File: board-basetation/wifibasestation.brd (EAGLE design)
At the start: 50 x 22 mm, 33 parts, among them IC1 1117EMP, IC2 HTU21D, J1 SWD_SHROUD_SMD, X1 ESP-03, X2 SMA-142-0711-821/826

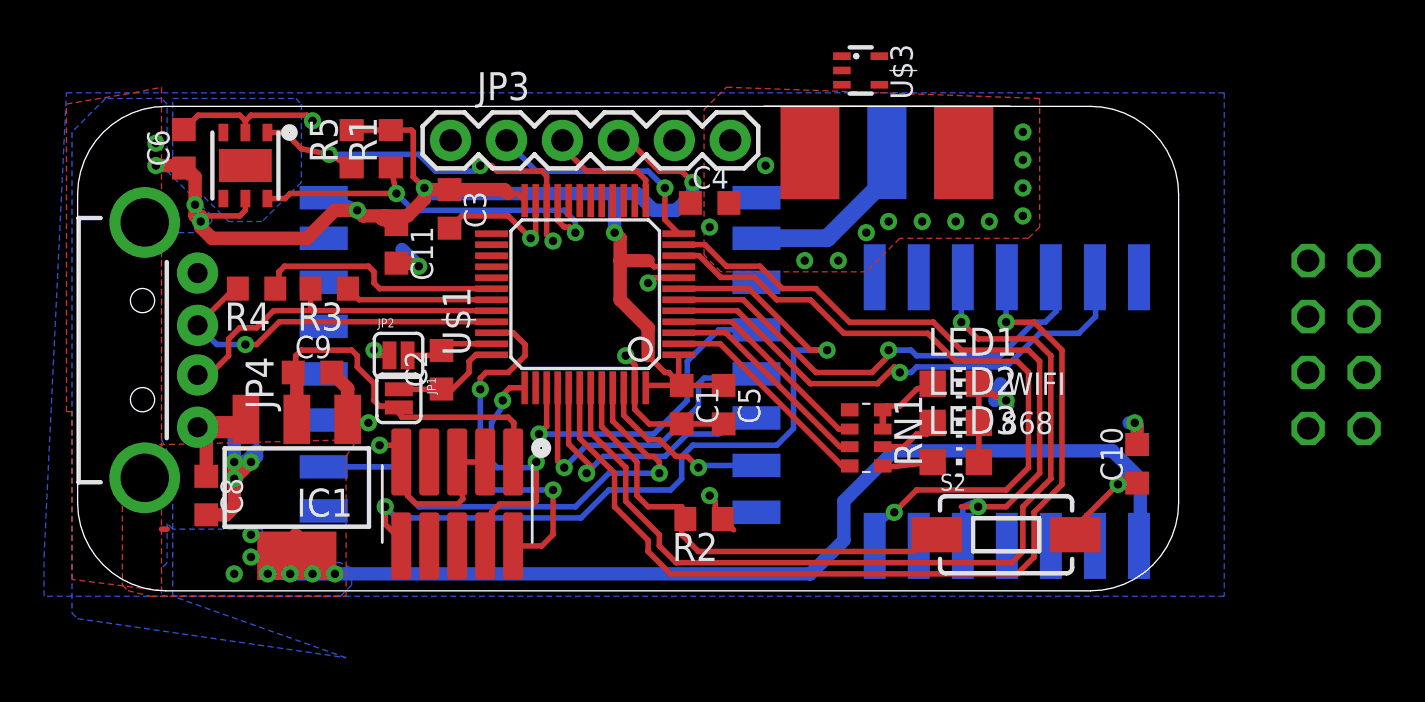
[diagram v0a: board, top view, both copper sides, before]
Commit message: pretty much done
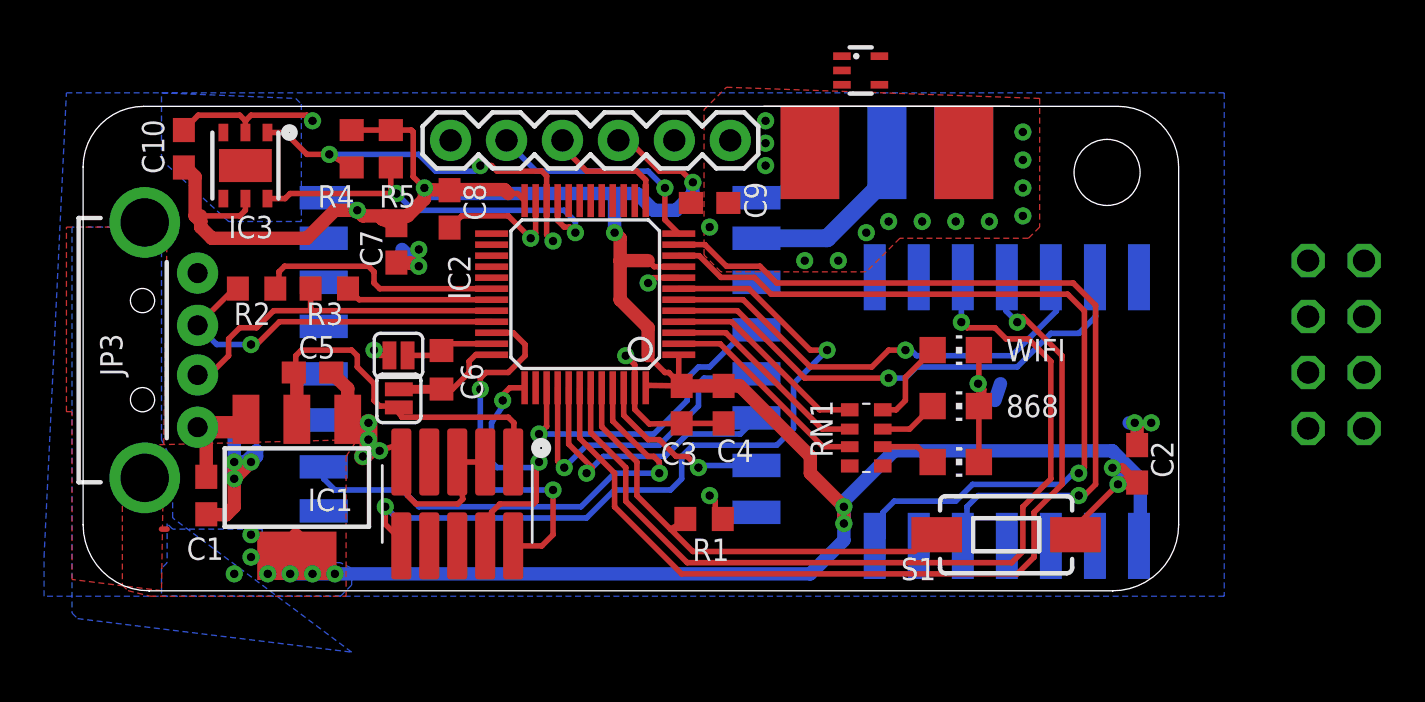
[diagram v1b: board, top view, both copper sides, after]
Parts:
- removed C11: (no value), rcl:C0603K
- removed U$3: LMT85, Mine:SC70-5L
- added C7: 1u, rcl:C0603
- added IC3: HTU21D, Mine:DFN6-L
- C1, C5: value (none) -> 4u7; device rcl:C0603K -> rcl:C0603
- C10, C2, C3: value (none) -> 1u; device rcl:C0603K -> rcl:C0603
- C4, C8, C9: value (none) -> 100n; device rcl:C0603K -> rcl:C0603
- C6: value (none) -> 100n
- IC2: value HTU21D -> STM32F072; device Mine:DFN6-L -> dtb:TQFP48
- JP3: value FTDI_BASICPTH -> USB-A-H; device SparkFun-Connectors:FTDI_BASIC -> SparkFun-Connectors:USB-A-H
- JP4: value USB-A-H -> FTDI_BASICPTH; device SparkFun-Connectors:USB-A-H -> SparkFun-Connectors:FTDI_BASIC
- R1, R2: value (none) -> 10k
- R3: value (none) -> 100k
- R4, R5: value (none) -> 4k7
- RN1: value (none) -> 330
- U$1: value STM32F072 -> LMT85; device dtb:TQFP48 -> Mine:SC70-5L
- moved C10 45.6 mm to (4.83, 20.6)
- moved C2 31.9 mm to (48.1, 6.27)
- moved R2 22.9 mm to (8.13, 14.2)
- moved R1 22.0 mm to (28.4, 3.76), turned to 180 degrees
- moved C1 22.0 mm to (5.84, 4.83)
- moved C9 19.6 mm to (28.7, 18.1)
- moved C5 18.7 mm to (10.7, 10.4), turned to 0 degrees
- moved C8 17.1 mm to (16.9, 17.8)
- moved JP3 16.8 mm to (3.05, 11.4)
- moved JP4 16.8 mm to (16.9, 21.0)
- moved IC2 16.5 mm to (23.1, 14.0), turned to 90 degrees
- moved U$1 16.1 mm to (35.6, 24.1), turned to 270 degrees
- moved C6 15.4 mm to (16.5, 10.5)
- moved C3 13.8 mm to (27.4, 8.95)
- moved C4 9.18 mm to (29.3, 8.95), turned to 270 degrees
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- renumbered S2 to S1
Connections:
- net +3V3: now also C2.1, C7.1, C8.1, IC2.1, IC2.24, IC2.48, IC2.9, IC3.5, JP4.VCC, R4.2; no longer C1.1, C11.1, C6.1, IC2.5, JP3.VCC, R1.2, U$1.1, U$1.24, U$1.48, U$1.9
- net CH_PD: now also IC2.5; no longer U$1.5
- net DIO0: now also IC2.45; no longer U$1.45
- net DM: now also IC2.32, JP3.D-; no longer JP4.D-, U$1.32
- net DP: now also IC2.33, JP3.D+, R2.2; no longer JP4.D+, R4.2, U$1.33
- net GND: now also C2.2, C7.2, IC2.23, IC2.47, IC2.8, IC3.2, R1.1; no longer C11.2, C6.2, IC2.2, R2.1, U$1.23, U$1.47, U$1.8
- net GPIO0: now also IC2.10; no longer U$1.10
- net GPIO15: now also IC2.11; no longer U$1.11
- net I2C2_SCL: now also IC2.21, IC3.6, R5.1; no longer IC2.6, R1.1, U$1.21
- net I2C2_SDA: now also IC2.22, IC3.1, R4.1; no longer IC2.1, R5.1, U$1.22
- net MISO: now also IC2.40; no longer U$1.40
- net MOSI: now also IC2.41; no longer U$1.41
- net N$10: now also RN1.7; no longer RN1.6
- net N$11: now also C6.1, IC2.36; no longer C2.1, U$1.36
- net N$12: now also IC2.15; no longer U$1.15
- net N$13: now also C6.2, IC2.35; no longer C2.2, U$1.35
- net N$14: now also IC2.16; no longer U$1.16
- net N$15: now also IC2.44, R1.2; no longer R2.2, U$1.44
- net N$16: now also IC2.17; no longer U$1.17
- net N$17: now also IC2.31; no longer U$1.31
- net N$18: now also IC2.30, R2.1; no longer R4.1, U$1.30
- net N$2: now also IC2.2, RN1.3; no longer RN1.4, U$1.2
- net N$20: now also LED1.A, RN1.6; no longer LED3.A, RN1.5
- net N$21: now also IC2.3, RN1.2; no longer RN1.3, U$1.3
- net N$22: now also IC2.4, RN1.1; no longer RN1.2, U$1.4
- net N$26: now also IC2.26; no longer U$1.26
- net N$27: now also IC2.27; no longer U$1.27
- net N$8: now also IC2.14; no longer U$1.14
- net N$9: now also LED3.A; no longer LED1.A, RN1.7
- net NRST: now also IC2.7; no longer U$1.7
- net NSS: now also IC2.46; no longer U$1.46
- net SCK: now also IC2.39; no longer U$1.39
- net SWCLK: now also IC2.37; no longer U$1.37
- net SWDAT: now also IC2.34; no longer U$1.34
- net USART1_RX: now also IC2.43; no longer U$1.43
- net USART1_TX: now also IC2.42; no longer U$1.42
- net USART2_RX: now also IC2.13, JP4.TXO; no longer JP3.TXO, U$1.13
- net USART2_TX: now also IC2.12, JP4.RXI; no longer JP3.RXI, U$1.12
- net VBUS: now also C1.1, JP3.VBUS; no longer C8.1, JP4.VBUS
- net W_RST: now also IC2.6; no longer U$1.6
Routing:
- net +3V3: track 137.8 -> 146.9 mm, vias 16 -> 15
- net GPIO0: track 31.3 -> 38.2 mm
- net GPIO15: track 30.4 -> 36.4 mm
- net GND: track 56.4 -> 58.4 mm, vias 27 -> 33
- net SCK: track 16.2 -> 14.7 mm
- net NRST: track 36.0 -> 35.1 mm
- net USART1_TX: track 42.0 -> 41.5 mm
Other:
- board size 50 x 22 mm -> 49.8 x 22 mm
- board text added: "IC3"
